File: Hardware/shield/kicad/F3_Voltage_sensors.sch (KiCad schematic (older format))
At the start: 19 parts, among them U1 MCP6244, U2 MCP6242

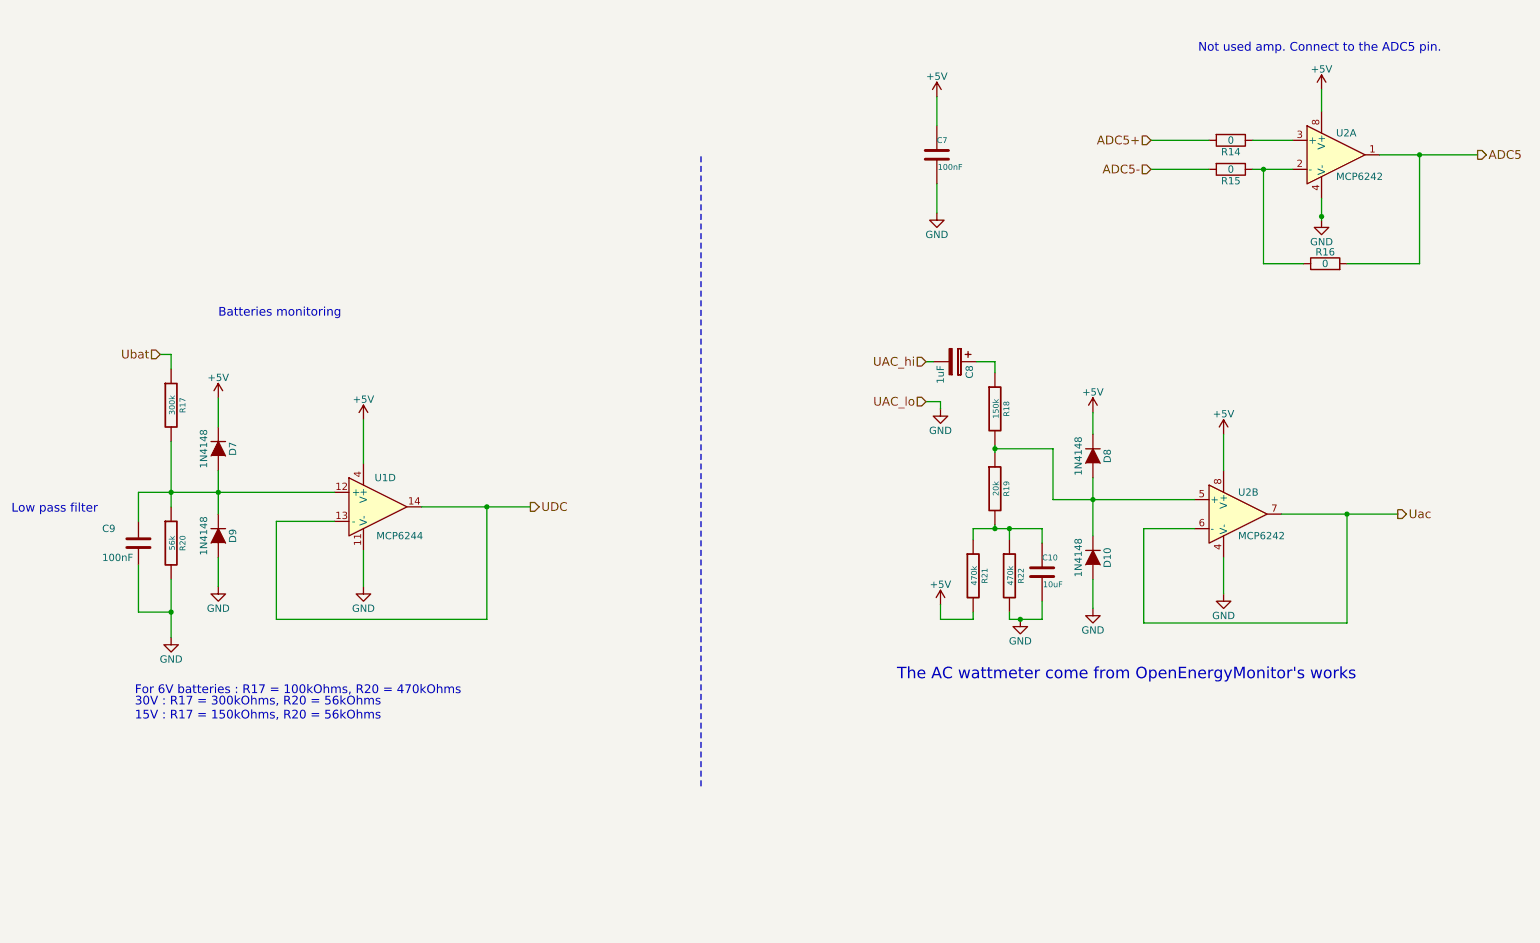
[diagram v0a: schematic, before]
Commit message: move to digital 1.1.1
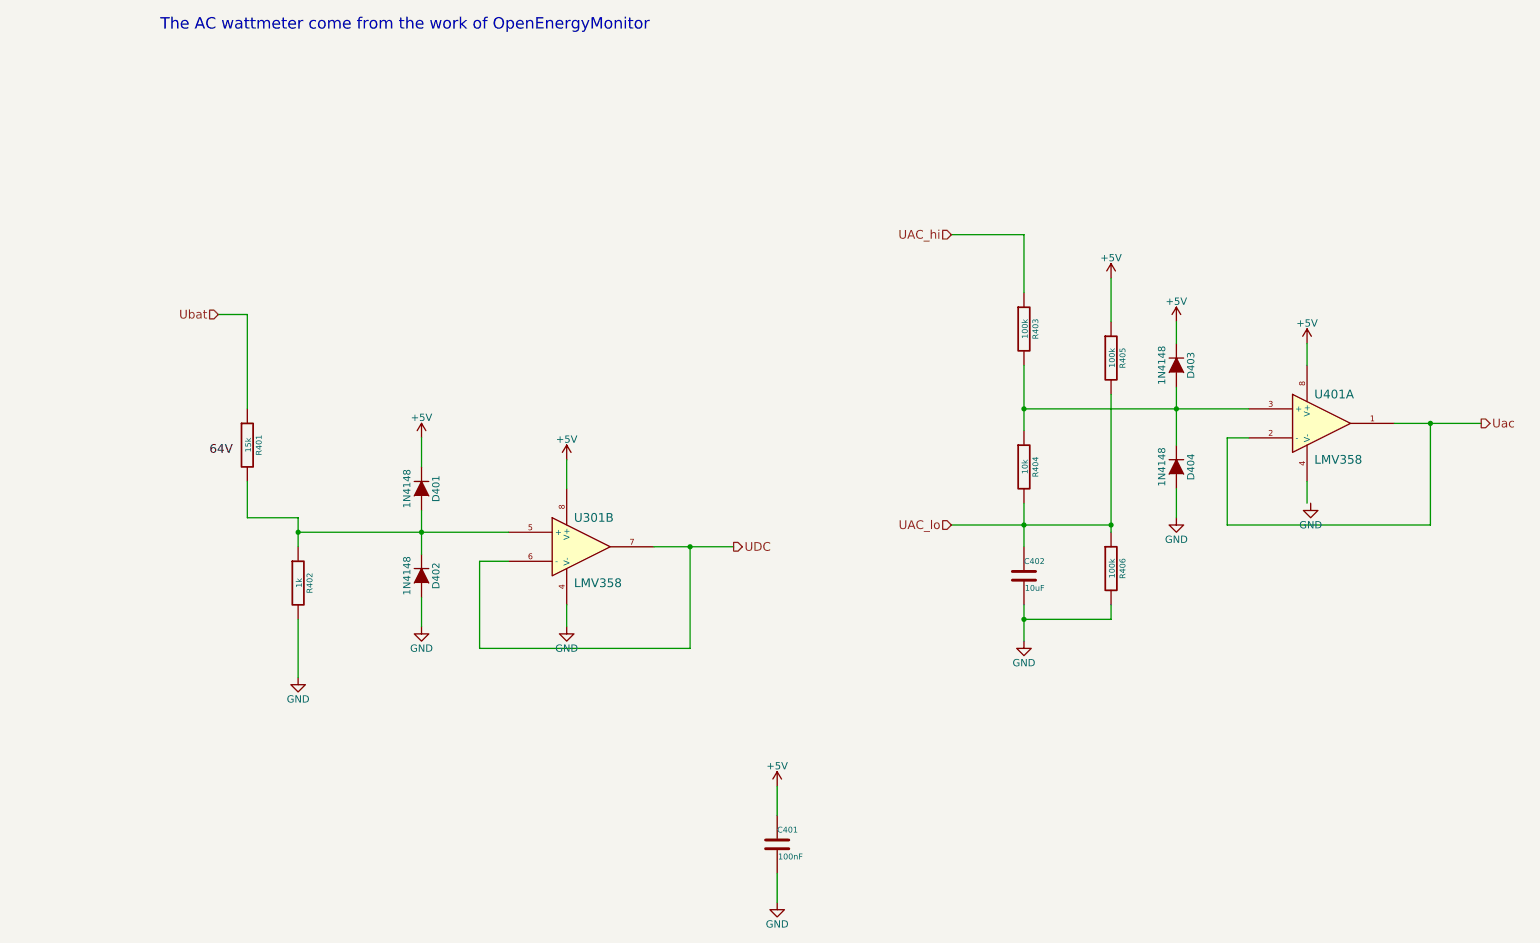
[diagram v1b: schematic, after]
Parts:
- removed C8: 1uF, Capacitors_ThroughHole:C_Radial_D5_L6_P2.5, symbol CP
- removed C9: 100nF, Capacitors_ThroughHole:C_Rect_L7_W2.5_P5, symbol C
- removed R14, R15, R16: 0, Discret:R3-LARGE_PADS, symbol R
- removed U1: MCP6244, Housings_DIP:DIP-14_W7.62mm_LongPads, symbol MCP6004
- removed U2: MCP6242, Housings_DIP:DIP-8_W7.62mm_LongPads, symbol MCP6002
- added U301, U401: LMV358, Housings_DIP:DIP-8_W7.62mm_LongPads, symbol LM358-RESCUE-Windlogger
- D401: renamed from D7; footprint Discret:DO-35 -> Diodes_ThroughHole:Diode_DO-35_SOD27_Horizontal_RM10
- D402: renamed from D9; footprint Discret:DO-35 -> Diodes_ThroughHole:Diode_DO-35_SOD27_Horizontal_RM10
- D403: renamed from D8; footprint Discret:DO-35 -> Diodes_ThroughHole:Diode_DO-35_SOD27_Horizontal_RM10
- D404: renamed from D10; footprint Discret:DO-35 -> Diodes_ThroughHole:Diode_DO-35_SOD27_Horizontal_RM10
- R401: renamed from R17; value 300k -> 15k; footprint Discret:R3-LARGE_PADS -> Discret:R4
- R402: renamed from R20; value 56k -> 1k; footprint Discret:R3-LARGE_PADS -> Discret:R4
- R403: renamed from R18; value 150k -> 100k; footprint Discret:R3-LARGE_PADS -> Discret:R4
- R404: renamed from R19; value 20k -> 10k; footprint Discret:R3-LARGE_PADS -> Discret:R4
- R405: renamed from R22; value 470k -> 100k; footprint Discret:R3-LARGE_PADS -> Discret:R4
- R406: renamed from R21; value 470k -> 100k; footprint Discret:R3-LARGE_PADS -> Discret:R4
- renumbered C7 to C401, C10 to C402
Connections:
- net +5V: now also R405.1, U301.8 (V+), U401.8 (V+); no longer R406.2
- net GND: now also R406.2, U301.4 (V-); no longer R405.2
- net UAC_hi: now also R403.1
- net UDC: now also U301.6 (-), U301.7
- net Uac: now also U401.1, U401.2 (-)
- net at D403.2 (A), D404.1 (K), R403.2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: now also U401.3 (+)
- net UAC_lo: now reaches C402.1, R404.2, R406.1
- net UAC_lo: now also R405.2; no longer R405.1
- net at D401.2 (A), D402.1 (K), R401.2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: now also U301.5 (+)
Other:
- note added: "The AC wattmeter come from the work of OpenEnergyMonitor"
- note removed: "30V : R17 = 300kOhms, R20 = 56kOhms\n15V : R17 = 150kOhms, R20 = 56kOhms"
- note removed: "Batteries monitoring"
- note removed: "For 6V batteries : R17 = 100kOhms, R20 = 470kOhms"
- note removed: "Low pass filter"
- note removed: "Not used amp. Connect to the ADC5 pin."
- note removed: "The AC wattmeter come from OpenEnergyMonitor's works"
- moved on the sheet: C401, C402, D401, D402, D403, D404, R401, R402, R403, R404, R405, R406
